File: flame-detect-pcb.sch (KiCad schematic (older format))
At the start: 48 parts, among them IC1 ATMEGA328-P, IC2 CH340G, Q1 MMBT2222, Q17 MMBT2222, Q2 MMBT2222, Q3 MMBT2907, Q4 MMBT2222, Q5 MMBT2907, Q6 MMBT2222, Q7 MMBT2222, T1 TRANSFORMER_(42TL013-RC), U1 NCV7805BDTRKG, X1 Crystal_GND2, X2 Crystal_GND2

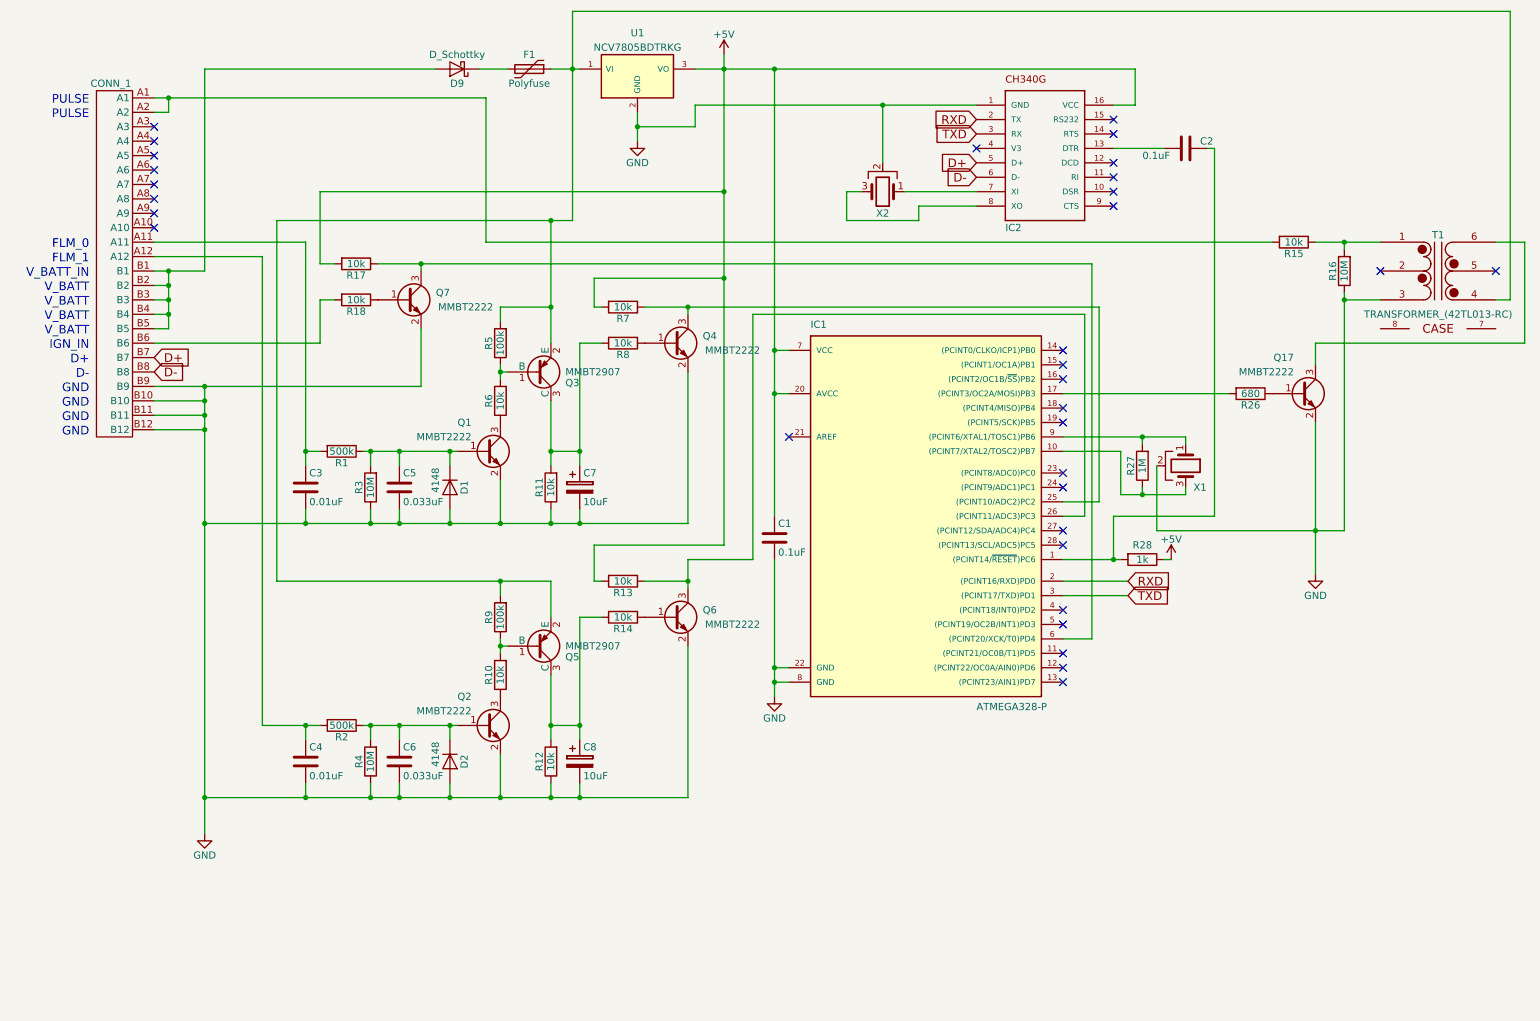
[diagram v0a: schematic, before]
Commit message: - Finished circuit for new 8 channel version.  Ready to start on PCB.
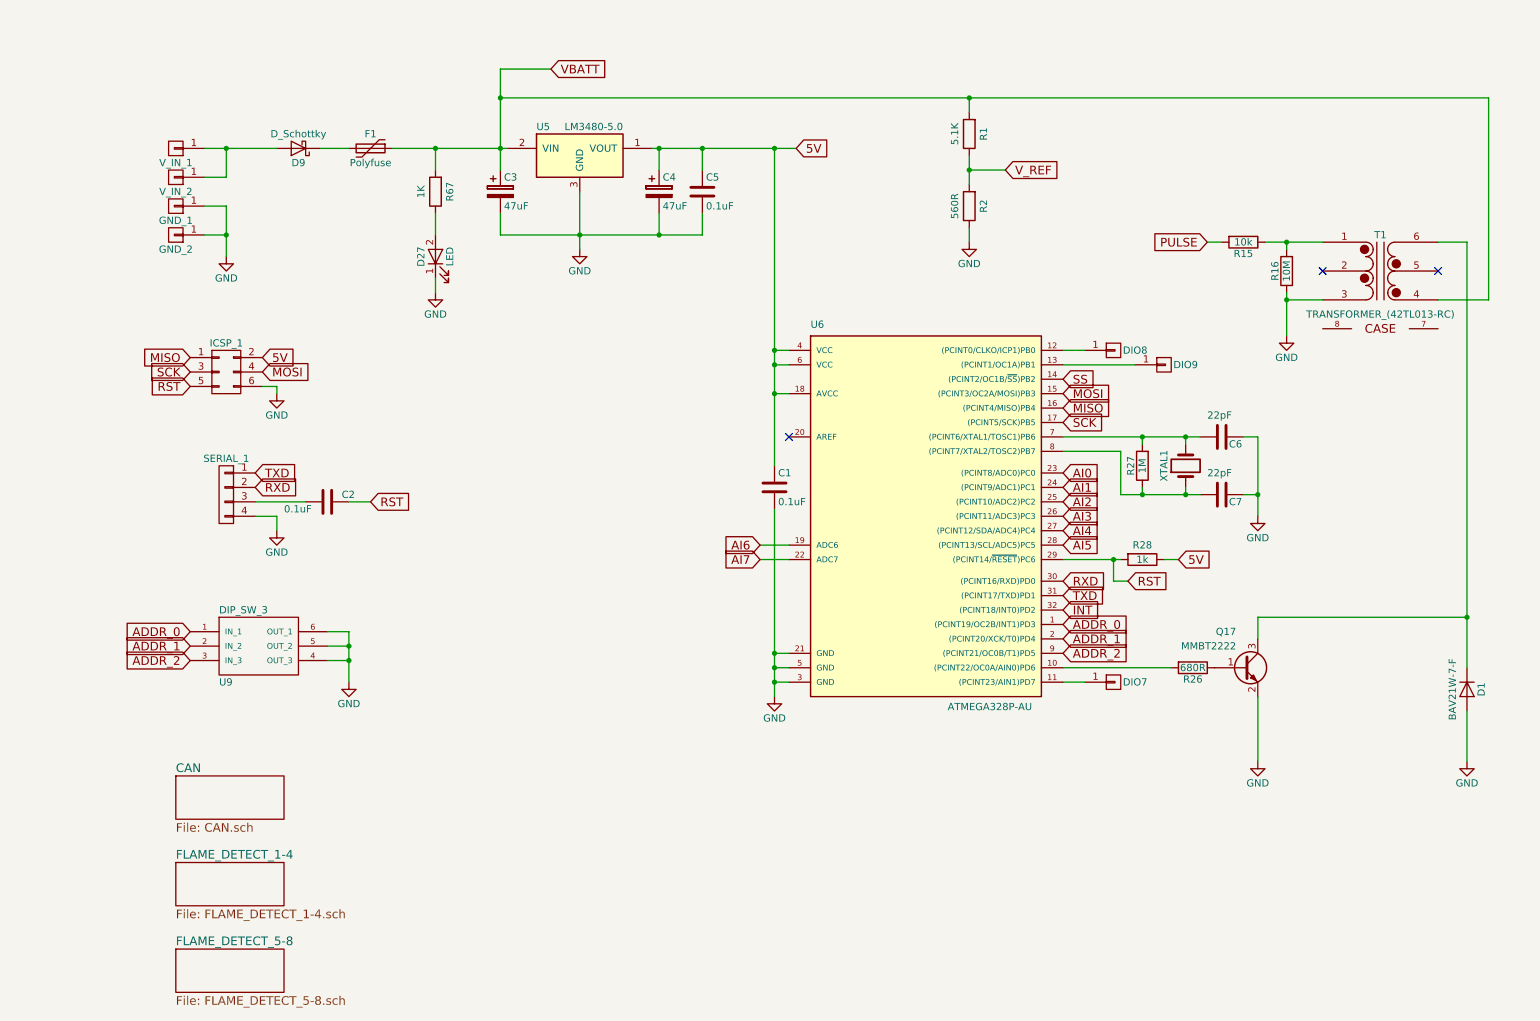
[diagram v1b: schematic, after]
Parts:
- removed C3, C4: 0.01uF, flame-detect-pcb:R_1206_HandSoldering_(narrow), symbol C
- removed C7, C8: 10uF, Capacitors_SMD:CP_Elec_4x4.5, symbol CP
- removed CONN_1: DEUTSCH_CONN_(DTM13-12PA-12PB-R008), flame-detect-pcb:DEUTSCH_CONN_(DTM13-12PA-12PB-R008), symbol DEUTSCH_CONN_(DTM13-12PA-12PB-R008)
- removed D2: 4148, Diodes_SMD:D_SOD-323_HandSoldering, symbol D
- removed IC1: ATMEGA328-P, Housings_DIP:DIP-28_W7.62mm_LongPads, symbol ATMEGA328-P
- removed IC2: CH340G, flame-detect-pcb:CH340G, symbol CH340G
- removed Q1, Q2, Q4, Q6, Q7: MMBT2222, TO_SOT_Packages_SMD:SOT-23_Handsoldering, symbol Q_NPN_BEC
- removed Q3, Q5: MMBT2907, TO_SOT_Packages_SMD:SOT-23_Handsoldering, symbol MMBT3906
- removed R10, R11, R12, R13, R14, R17, R18, R6, R7, R8: 10k, flame-detect-pcb:R_1206_HandSoldering_(narrow), symbol R
- removed R3, R4: 10M, flame-detect-pcb:R_1206_HandSoldering_(narrow), symbol R
- removed R5, R9: 100k, flame-detect-pcb:R_1206_HandSoldering_(narrow), symbol R
- removed U1: NCV7805BDTRKG, flame-detect-pcb:REGULATOR_(NCV7805BDTRKG), symbol NCV7805BDTRKG
- removed X1, X2: Crystal_GND2, flame-detect-pcb:RESONATOR_(CSTCE16M0V53C-R0), symbol Crystal_GND2
- added C3, C4: 47uF, Capacitors_SMD:C_0805, symbol CP
- added C7: 22pF, Capacitors_SMD:C_0805, symbol C
- added D27: LED, symbol LED
- added DIO7, DIO8, DIO9, GND_1, GND_2, V_IN_1, V_IN_2: CONN_01X01, symbol CONN_01X01
- added ICSP_1: CONN_02X03, symbol CONN_02X03
- added R67: 1K, Resistors_SMD:R_0805, symbol R
- added SERIAL_1: CONN_01X04, symbol CONN_01X04
- added U5: LM3480-5.0, TO_SOT_Packages_SMD:SOT-23, symbol LM3480-5.0
- added U6: ATMEGA328P-AU, TQFP32, symbol ATMEGA328P-AU
- added U9: DIP_SW_3, symbol DIP_SW_3
- added XTAL1: Crystal, symbol Crystal
- C1, C2: footprint flame-detect-pcb:R_1206_HandSoldering_(narrow) -> Capacitors_SMD:C_0805
- C5: value 0.033uF -> 0.1uF; footprint flame-detect-pcb:R_1206_HandSoldering_(narrow) -> Capacitors_SMD:C_0805
- C6: value 0.033uF -> 22pF; footprint flame-detect-pcb:R_1206_HandSoldering_(narrow) -> Capacitors_SMD:C_0805
- D1: value 4148 -> BAV21W-7-F; footprint Diodes_SMD:D_SOD-323_HandSoldering -> Diodes_SMD:D_0805
- F1: footprint Resistors_SMD:R_1812_HandSoldering -> Resistors_SMD:R_1812
- Q17: footprint TO_SOT_Packages_SMD:SOT-23_Handsoldering -> TO_SOT_Packages_SMD:SOT-23
- R1: value 500k -> 5.1K; footprint flame-detect-pcb:R_1206_HandSoldering_(narrow) -> Resistors_SMD:R_0805
- R15, R16, R27, R28: footprint flame-detect-pcb:R_1206_HandSoldering_(narrow) -> Resistors_SMD:R_0805
- R2: value 500k -> 560R; footprint flame-detect-pcb:R_1206_HandSoldering_(narrow) -> Resistors_SMD:R_0805
- R26: value 680 -> 680R; footprint flame-detect-pcb:R_1206_HandSoldering_(narrow) -> Resistors_SMD:R_0805
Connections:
- net GND: now also C6.1, R2.1, C3.2, C4.2, C7.1, D27.1 (K), GND_1.1 (P1), GND_2.1 (P1), ICSP_1.6 (P6), SERIAL_1.4 (P4), U5.3 (GND), U6.21 (GND), U6.3 (GND), U6.5 (GND), U9.4 (OUT_3), U9.5 (OUT_2), U9.6 (OUT_1); no longer C6.2
- net RXD: now also SERIAL_1.2 (P2), U6.30 ((PCINT16/RXD)PD0)
- net TXD: now also SERIAL_1.1 (P1), U6.31 ((PCINT17/TXD)PD1)
- net at Q17.3 (C), T1.6 (S3): now also D1.1 (K)
- net at R26.2: now also U6.10 ((PCINT22/OC0A/AIN0)PD6)
- net PULSE: now reaches R15.2
- net VBATT: now reaches R1.2
- net VBATT: now also F1.1, T1.4 (S1), C3.1, R67.2, U5.2 (VIN)
- net V_REF: now reaches R2.2
- net V_REF: now also R1.1
- net at D9.2 (A): now also V_IN_1.1 (P1), V_IN_2.1 (P1)
- net RST: now reaches C2.1, R28.2
- net RST: now also ICSP_1.5 (P5), U6.29 ((PCINT14/~RESET~)PC6)
- net at R27.1: now also C7.2, U6.8 ((PCINT7/XTAL2/TOSC2)PB7), XTAL1.1
- net at R27.2: now also C6.2, U6.7 ((PCINT6/XTAL1/TOSC1)PB6), XTAL1.2
- net at C2.2: now also SERIAL_1.3 (P3)
- net +5V renamed 5V
- net 5V: now also C5.1, C4.1, ICSP_1.2 (P2), U5.1 (VOUT), U6.18 (AVCC), U6.4 (VCC), U6.6 (VCC)
- new net: DIO7.1 (P1), U6.11 ((PCINT23/AIN1)PD7)
- new net: DIO8.1 (P1), U6.12 ((PCINT0/CLKO/ICP1)PB0)
- new net: DIO9.1 (P1), U6.13 ((PCINT1/OC1A)PB1)
- new net: D27.2 (A), R67.1
- new net ADDR_0: U6.1 ((PCINT19/OC2B/INT1)PD3), U9.1 (IN_1)
- new net ADDR_1: U6.2 ((PCINT20/XCK/T0)PD4), U9.2 (IN_2)
- new net ADDR_2: U6.9 ((PCINT21/OC0B/T1)PD5), U9.3 (IN_3)
- new net AI0: U6.23 ((PCINT8/ADC0)PC0)
- new net AI1: U6.24 ((PCINT9/ADC1)PC1)
- new net AI2: U6.25 ((PCINT10/ADC2)PC2)
- new net AI3: U6.26 ((PCINT11/ADC3)PC3)
- new net AI4: U6.27 ((PCINT12/SDA/ADC4)PC4)
- new net AI5: U6.28 ((PCINT13/SCL/ADC5)PC5)
- new net AI6: U6.19 (ADC6)
- new net AI7: U6.22 (ADC7)
- new net INT: U6.32 ((PCINT18/INT0)PD2)
- new net MISO: ICSP_1.1 (P1), U6.16 ((PCINT4/MISO)PB4)
- new net MOSI: ICSP_1.4 (P4), U6.15 ((PCINT3/OC2A/MOSI)PB3)
- new net SCK: ICSP_1.3 (P3), U6.17 ((PCINT5/SCK)PB5)
- new net SS: U6.14 ((PCINT2/OC1B/~SS~)PB2)
- no-connect marks 32 -> 3
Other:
- note removed: "D+"
- note removed: "D-"
- note removed: "FLM_0"
- note removed: "FLM_1"
- note removed: "GND"
- note removed: "IGN_IN"
- note removed: "PULSE"
- note removed: "V_BATT"
- note removed: "V_BATT_IN"
- moved on the sheet: C1, C2, D9, F1, Q17, R15, R16, R26, T1

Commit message: - Finished footprints.
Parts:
- D1: footprint Diodes_SMD:D_0805 -> Diodes_SMD:D_SOD-123
- D27: footprint (none) -> LEDs:LED_1206
- DIO7, DIO8, DIO9: footprint (none) -> flame-detect-pcb:SPARE_THROUGH_HOLE
- GND_1, GND_2, V_IN_1, V_IN_2: footprint (none) -> flame-detect-pcb:KEYSTONE_SPADE_TERM_(1287)
- ICSP_1: footprint (none) -> Pin_Headers:Pin_Header_Straight_2x03_Pitch2.54mm_SMD
- SERIAL_1: footprint (none) -> Pin_Headers:Pin_Header_Straight_1x04_Pitch2.54mm_SMD_Pin1Left
- U6: footprint TQFP32 -> Housings_QFP:TQFP-32_7x7mm_Pitch0.8mm
- U9: footprint (none) -> Buttons_Switches_SMD:SW_DIP_x3_W8.61mm_Slide_LowProfile
- XTAL1: footprint (none) -> Crystals:Crystal_SMD_HC49-SD
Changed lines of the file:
@@
 F 0 "U6" H 6000 5250 50  0000 L BNN
 F 1 "ATMEGA328P-AU" H 6950 2600 50  0000 L BNN
-F 2 "TQFP32" H 6750 4000 50  0001 C CIN
+F 2 "Housings_QFP:TQFP-32_7x7mm_Pitch0.8mm" H 6750 4000 50  0001 C CIN
 F 3 "" H 6750 4000 50  0001 C CNN
 	1    6750 4000
@@
 F 0 "V_IN_1" H 1600 1600 50  0000 C CNN
 F 1 "CONN_01X01" V 1700 1500 50  0001 C CNN
-F 2 "" H 1600 1500 50  0001 C CNN
+F 2 "flame-detect-pcb:KEYSTONE_SPADE_TERM_(1287)" H 1600 1500 50  0001 C CNN
 F 3 "" H 1600 1500 50  0001 C CNN
 	1    1600 1500
@@
 F 0 "V_IN_2" H 1600 1800 50  0000 C CNN
 F 1 "CONN_01X01" V 1700 1700 50  0001 C CNN
-F 2 "" H 1600 1700 50  0001 C CNN
+F 2 "flame-detect-pcb:KEYSTONE_SPADE_TERM_(1287)" H 1600 1700 50  0001 C CNN
 F 3 "" H 1600 1700 50  0001 C CNN
 	1    1600 1700
@@
 F 0 "GND_1" H 1600 2000 50  0000 C CNN
 F 1 "CONN_01X01" V 1700 1900 50  0001 C CNN
-F 2 "" H 1600 1900 50  0001 C CNN
+F 2 "flame-detect-pcb:KEYSTONE_SPADE_TERM_(1287)" H 1600 1900 50  0001 C CNN
 F 3 "" H 1600 1900 50  0001 C CNN
 	1    1600 1900
@@
 F 0 "GND_2" H 1600 2200 50  0000 C CNN
 F 1 "CONN_01X01" V 1700 2100 50  0001 C CNN
-F 2 "" H 1600 2100 50  0001 C CNN
+F 2 "flame-detect-pcb:KEYSTONE_SPADE_TERM_(1287)" H 1600 2100 50  0001 C CNN
 F 3 "" H 1600 2100 50  0001 C CNN
 	1    1600 2100
@@
 F 0 "ICSP_1" H 1950 3250 50  0000 C CNN
 F 1 "CONN_02X03" H 1950 2850 50  0001 C CNN
-F 2 "" H 1950 1850 50  0001 C CNN
+F 2 "Pin_Headers:Pin_Header_Straight_2x03_Pitch2.54mm_SMD" H 1950 1850 50  0001 C CNN
 F 3 "" H 1950 1850 50  0001 C CNN
 	1    1950 3050
@@
 F 0 "SERIAL_1" H 1950 4150 50  0000 C CNN
 F 1 "CONN_01X04" V 2050 3900 50  0001 C CNN
-F 2 "" H 1950 3900 50  0001 C CNN
+F 2 "Pin_Headers:Pin_Header_Straight_1x04_Pitch2.54mm_SMD_Pin1Left" H 1950 3900 50  0001 C CNN
 F 3 "" H 1950 3900 50  0001 C CNN
 	1    1950 3900
@@
 F 0 "XTAL1" H 8600 3850 50  0000 C CNN
 F 1 "Crystal" H 8600 3550 50  0001 C CNN
-F 2 "" H 8600 3700 50  0001 C CNN
+F 2 "Crystals:Crystal_SMD_HC49-SD" H 8600 3700 50  0001 C CNN
 F 3 "" H 8600 3700 50  0001 C CNN
 	1    8600 3700
@@
 F 0 "D1" H 10550 5350 50  0000 C CNN
 F 1 "BAV21W-7-F" H 10550 5150 50  0000 C CNN
-F 2 "Diodes_SMD:D_0805" H 10550 5250 50  0001 C CNN
+F 2 "Diodes_SMD:D_SOD-123" H 10550 5250 50  0001 C CNN
 F 3 "" H 10550 5250 50  0001 C CNN
 	1    10550 5250
@@
 F 0 "DIO8" H 8250 2900 50  0000 C CNN
 F 1 "CONN_01X01" V 8200 2900 50  0001 C CNN
-F 2 "" H 8100 2900 50  0001 C CNN
+F 2 "flame-detect-pcb:SPARE_THROUGH_HOLE" H 8100 2900 50  0001 C CNN
 F 3 "" H 8100 2900 50  0001 C CNN
 	1    8100 2900
@@
 F 0 "DIO9" H 8600 3000 50  0000 C CNN
 F 1 "CONN_01X01" V 8550 3000 50  0001 C CNN
-F 2 "" H 8450 3000 50  0001 C CNN
+F 2 "flame-detect-pcb:SPARE_THROUGH_HOLE" H 8450 3000 50  0001 C CNN
 F 3 "" H 8450 3000 50  0001 C CNN
 	1    8450 3000
@@
 F 0 "DIO7" H 8250 5200 50  0000 C CNN
 F 1 "CONN_01X01" V 8200 5200 50  0001 C CNN
-F 2 "" H 8100 5200 50  0001 C CNN
+F 2 "flame-detect-pcb:SPARE_THROUGH_HOLE" H 8100 5200 50  0001 C CNN
 F 3 "" H 8100 5200 50  0001 C CNN
 	1    8100 5200
@@
 F 0 "U9" H 1900 4700 50  0000 L CNN
 F 1 "DIP_SW_3" H 1900 5200 50  0000 L CNN
-F 2 "" H 1900 4600 50  0001 L CNN
+F 2 "Buttons_Switches_SMD:SW_DIP_x3_W8.61mm_Slide_LowProfile" H 1900 4600 50  0001 L CNN
 F 3 "" H 2300 4600 60  0001 C CNN
 	1    2150 4950
@@
 F 0 "D27" H 3400 2350 50  0000 C CNN
 F 1 "LED" H 3400 2150 50  0000 C CNN
-F 2 "" H 3400 2250 50  0001 C CNN
+F 2 "LEDs:LED_1206" H 3400 2250 50  0001 C CNN
 F 3 "" H 3400 2250 50  0001 C CNN
 	1    3400 2250
